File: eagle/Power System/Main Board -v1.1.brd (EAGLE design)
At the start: 101.6 x 100 mm, 19 parts

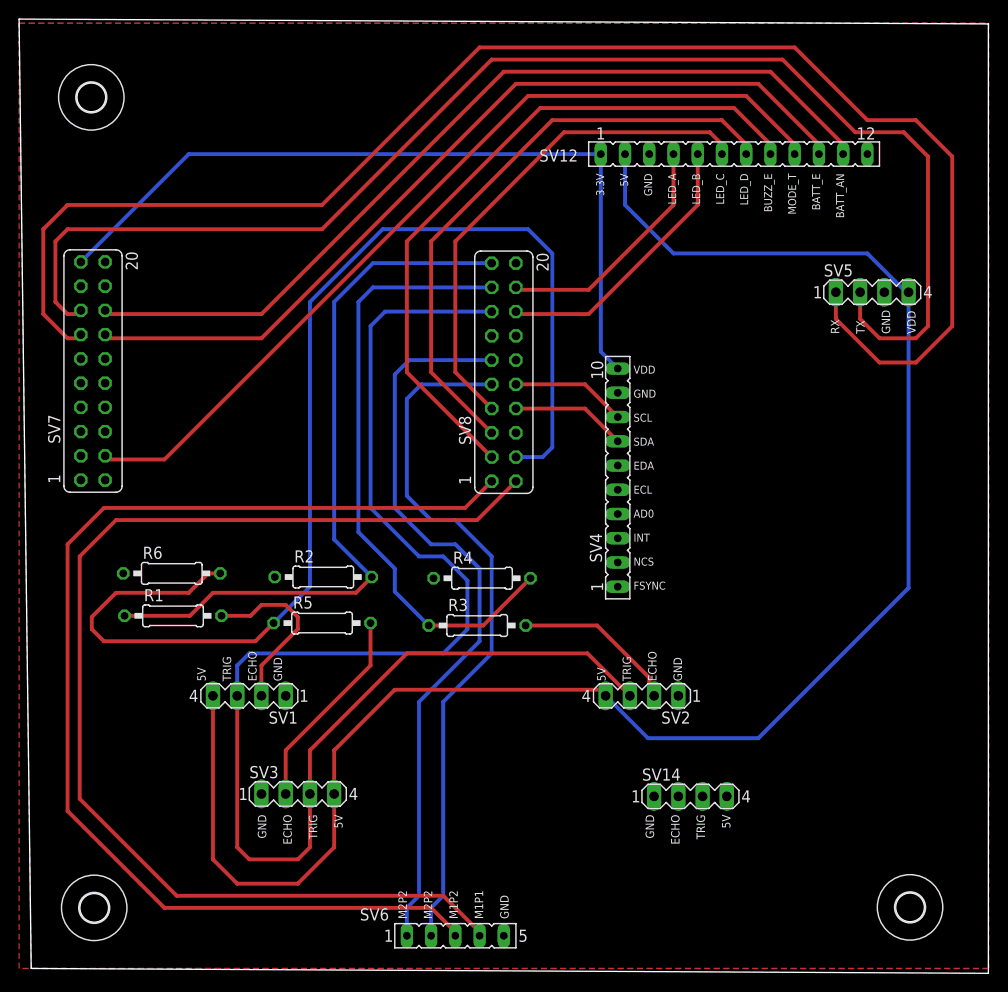
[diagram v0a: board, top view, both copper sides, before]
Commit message: final final final eagle files
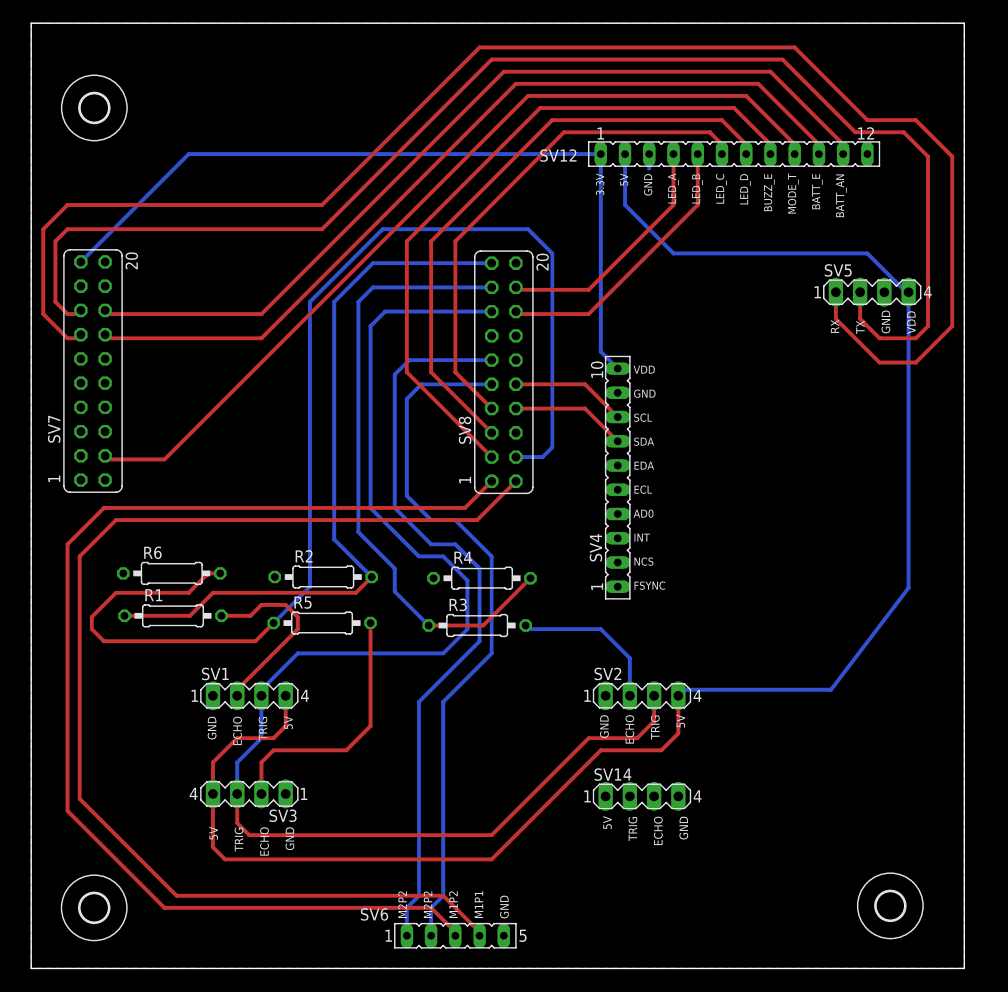
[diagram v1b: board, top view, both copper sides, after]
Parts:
- moved SV3 5.08 mm to (25.4, 22.1), turned to 180 degrees
- moved SV14 5.08 mm to (66.5, 21.8)
- moved U$2 2.07 mm to (92.6, 10.4)
- moved U$1 1.16 mm to (9.16, 94.0)
- turned SV1 to 0 degrees
- turned SV2 to 0 degrees
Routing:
- net N$24: track 153.9 -> 141.8 mm
- net N$17: track 21.6 -> 27.1 mm
- net +5V: track 183.3 -> 178.9 mm
- net N$3: track 0.00 -> 1.27 mm
- net N$1: track 18.8 -> 19.9 mm
- net N$7: track 17.3 -> 16.3 mm
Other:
- board size 101.6 x 100 mm -> 97.8 x 99.1 mm

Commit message: added multimeter
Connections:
- new net N$2: SV12.12, SV7.12
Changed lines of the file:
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@@
 <wire x1="67.31" y1="87.63" x2="67.31" y2="88.9" width="0.4064" layer="16"/>
+</signal>
+<signal name="N$2">
+<contactref element="SV12" pad="12"/>
+<contactref element="SV7" pad="12"/>
+<wire x1="10.287" y1="67.691" x2="90.17" y2="89.154" width="0" layer="19" extent="1-1"/>
 </signal>
 </signals>
